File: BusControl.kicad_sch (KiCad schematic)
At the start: 29 parts, among them U17 74LVC74AD, U18 74LVC74AD, U19 74LVC74AD, U20 74LVC86AD, U21 74LVC32AD, U22 74LVC02AD, U23 74LVC00AD, U24 74LVC125AD, U25 74LVC32AD, U26 74LVC125AD, U34 74LVC32AD, U35 74LVC74AD, U36 74LVC74AD, U37 74LVC74AD, U42 74LVC32AD

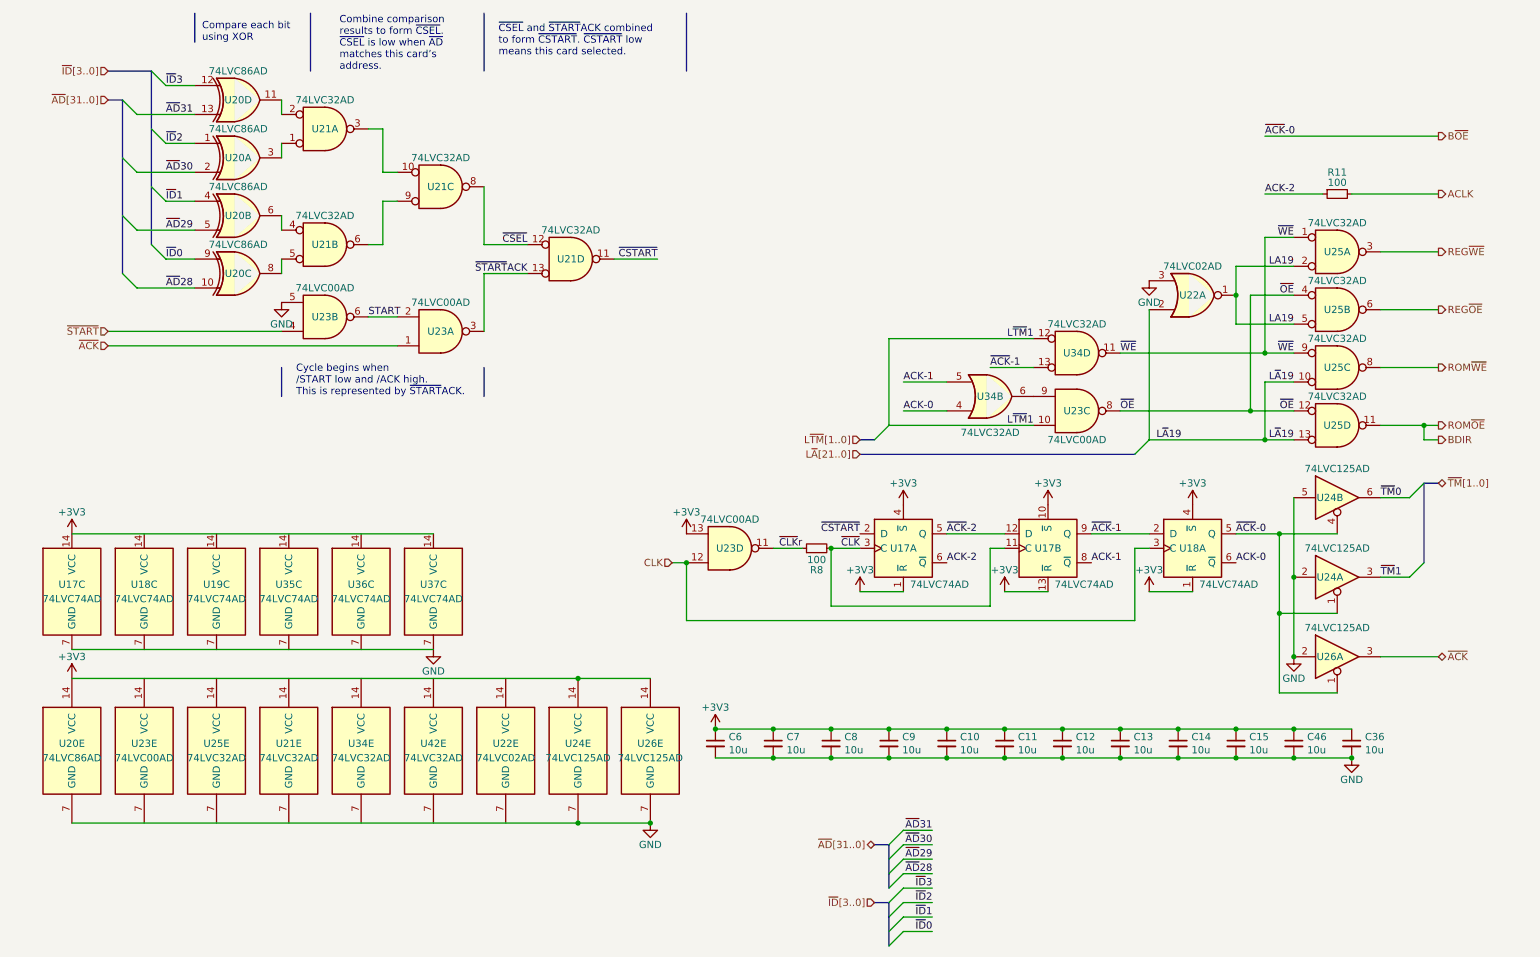
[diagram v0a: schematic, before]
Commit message: Revert "did I mess this up?"
This reverts commit fd75c937204418059e97b488ea791750328fc4dd.
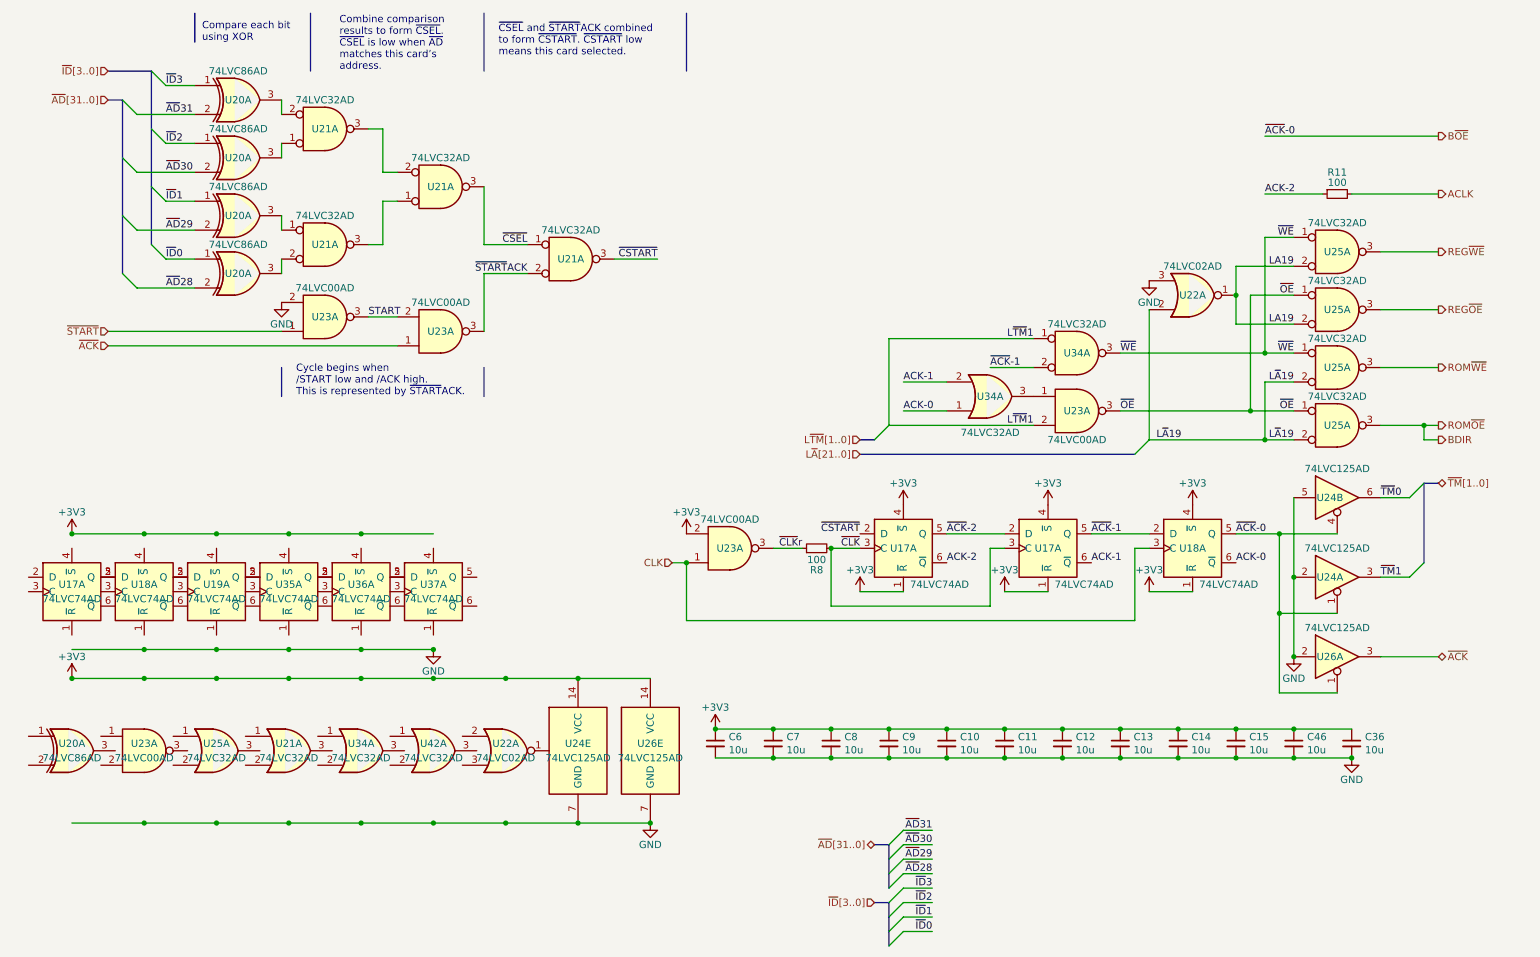
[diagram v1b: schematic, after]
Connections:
- net +3V3: now also U17.1 (~{R}), U17.4 (~{S}), U23.2; no longer U17.10 (~{S}), U17.13 (~{R}), U17.14 (VCC), U20.14 (VCC), U23.13, U37.14 (VCC)
- net ACK-0: now also U34.1; no longer U34.4
- net ACK-1: now also U17.6 (~{Q}), U34.2; no longer U17.8 (~{Q}), U34.5
- net BDIR: now also U25.3; no longer U25.11
- net CLK: now also U23.1; no longer U23.12
- net GND: now also U23.2; no longer U17.7 (GND), U20.7 (GND), U23.5, U37.7 (GND)
- net LA19: now also U25.2; no longer U25.5
- net L~{A}19: now also U25.2, U25.2; no longer U25.10, U25.13
- net L~{TM}1: now also U23.2, U34.1; no longer U23.10, U34.12
- net REG~{OE}: now also U25.3; no longer U25.6
- net ROM~{WE}: now also U25.3; no longer U25.8
- net START: now also U23.3; no longer U23.6
- net ~{ACK}-1: now also U17.5 (Q), U34.2; no longer U17.9 (Q), U34.13
- net ~{ACK}-2: now also U17.2 (D); no longer U17.12 (D)
- net ~{AD}28: now also U20.2; no longer U20.10
- net ~{AD}29: now also U20.2; no longer U20.5
- net ~{AD}31: now also U20.2; no longer U20.13
- net ~{CLK}: now also U17.3 (C); no longer U17.11 (C)
- net ~{CLK}r: now also U23.3; no longer U23.11
- net ~{CSEL}: now also U21.1, U21.3; no longer U21.12, U21.8
- net ~{CSTART}: now also U21.3; no longer U21.11
- net ~{ID}0: now also U20.1; no longer U20.9
- net ~{ID}1: now also U20.1; no longer U20.4
- net ~{ID}3: now also U20.1; no longer U20.12
- net ~{OE}: now also U23.3, U25.1, U25.1; no longer U23.8, U25.12, U25.4
- net ~{START}: now also U23.1; no longer U23.4
- net ~{START}ACK: now also U21.2; no longer U21.13
- net ~{WE}: now also U25.1, U34.3; no longer U25.9, U34.11
- net at U21.3: now also U21.2; no longer U21.10
- net at U21.2: now also U20.3; no longer U20.11
- new net: U23.1, U34.3
- new net: U21.1, U21.3
- new net: U20.3, U21.1
- new net: U20.3, U21.2

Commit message: did I mess this up?
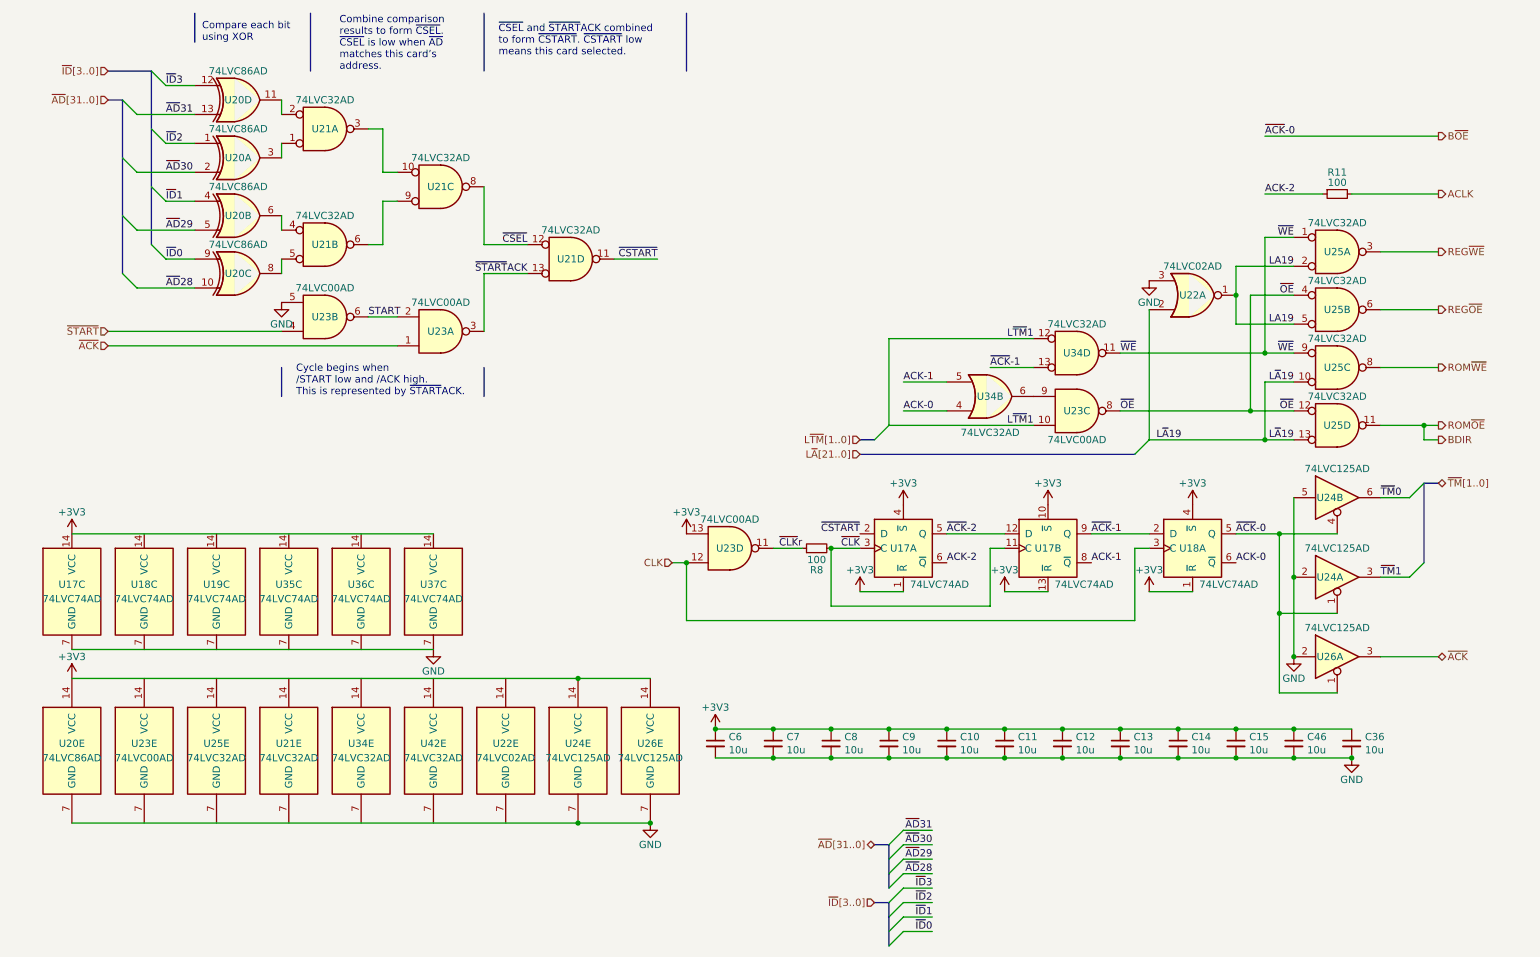
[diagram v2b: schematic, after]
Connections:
- net +3V3: now also U17.10 (~{S}), U17.13 (~{R}), U17.14 (VCC), U20.14 (VCC), U23.13, U37.14 (VCC); no longer U17.1 (~{R}), U17.4 (~{S}), U23.2
- net ACK-0: now also U34.4; no longer U34.1
- net ACK-1: now also U17.8 (~{Q}), U34.5; no longer U17.6 (~{Q}), U34.2
- net BDIR: now also U25.11; no longer U25.3
- net CLK: now also U23.12; no longer U23.1
- net GND: now also U17.7 (GND), U20.7 (GND), U23.5, U37.7 (GND); no longer U23.2
- net LA19: now also U25.5; no longer U25.2
- net L~{A}19: now also U25.10, U25.13; no longer U25.2, U25.2
- net L~{TM}1: now also U23.10, U34.12; no longer U23.2, U34.1
- net REG~{OE}: now also U25.6; no longer U25.3
- net ROM~{WE}: now also U25.8; no longer U25.3
- net START: now also U23.6; no longer U23.3
- net ~{ACK}-1: now also U17.9 (Q), U34.13; no longer U17.5 (Q), U34.2
- net ~{ACK}-2: now also U17.12 (D); no longer U17.2 (D)
- net ~{AD}28: now also U20.10; no longer U20.2
- net ~{AD}29: now also U20.5; no longer U20.2
- net ~{AD}31: now also U20.13; no longer U20.2
- net ~{CLK}: now also U17.11 (C); no longer U17.3 (C)
- net ~{CLK}r: now also U23.11; no longer U23.3
- net ~{CSEL}: now also U21.12, U21.8; no longer U21.1, U21.3
- net ~{CSTART}: now also U21.11; no longer U21.3
- net ~{ID}0: now also U20.9; no longer U20.1
- net ~{ID}1: now also U20.4; no longer U20.1
- net ~{ID}3: now also U20.12; no longer U20.1
- net ~{OE}: now also U23.8, U25.12, U25.4; no longer U23.3, U25.1, U25.1
- net ~{START}: now also U23.4; no longer U23.1
- net ~{START}ACK: now also U21.13; no longer U21.2
- net ~{WE}: now also U25.9, U34.11; no longer U25.1, U34.3
- net at U21.3: now also U21.10; no longer U21.2
- net at U21.2: now also U20.11; no longer U20.3
- new net: U23.9, U34.6
- new net: U21.6, U21.9
- new net: U20.6, U21.4
- new net: U20.8, U21.5
